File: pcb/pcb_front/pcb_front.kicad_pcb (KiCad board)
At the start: 2 copper layers, 30 x 27 mm, 24 parts, among them J1 MicroLab, J2 LED_BREAKOUT, J3 GAS_BREAKOUT, U1 TBD62783A

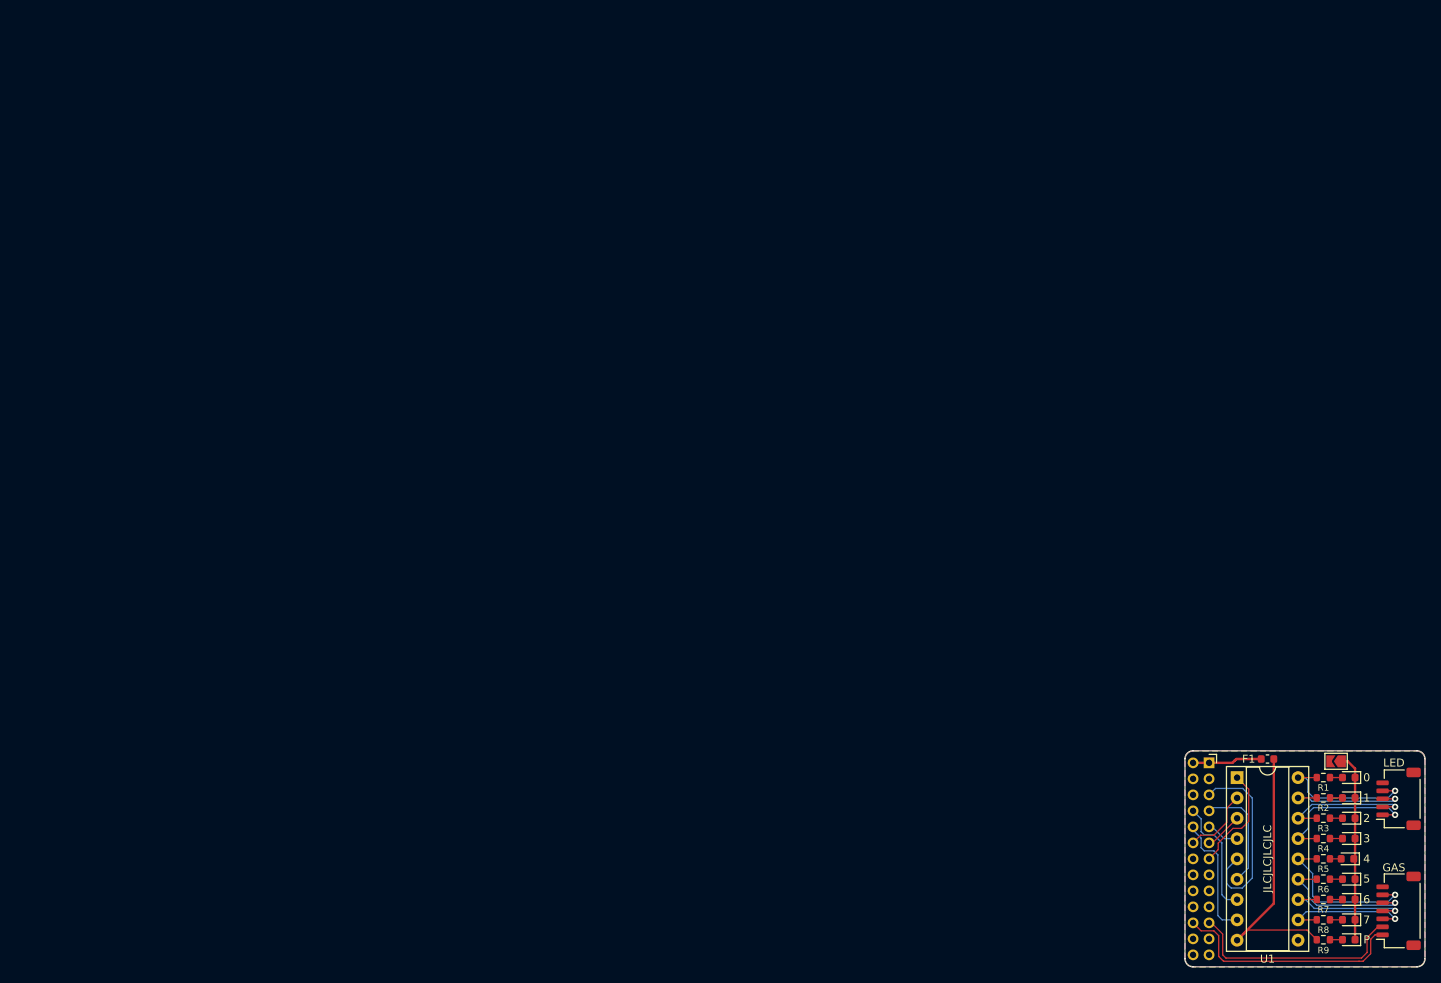
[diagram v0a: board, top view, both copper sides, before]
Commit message: front pcb rev 2
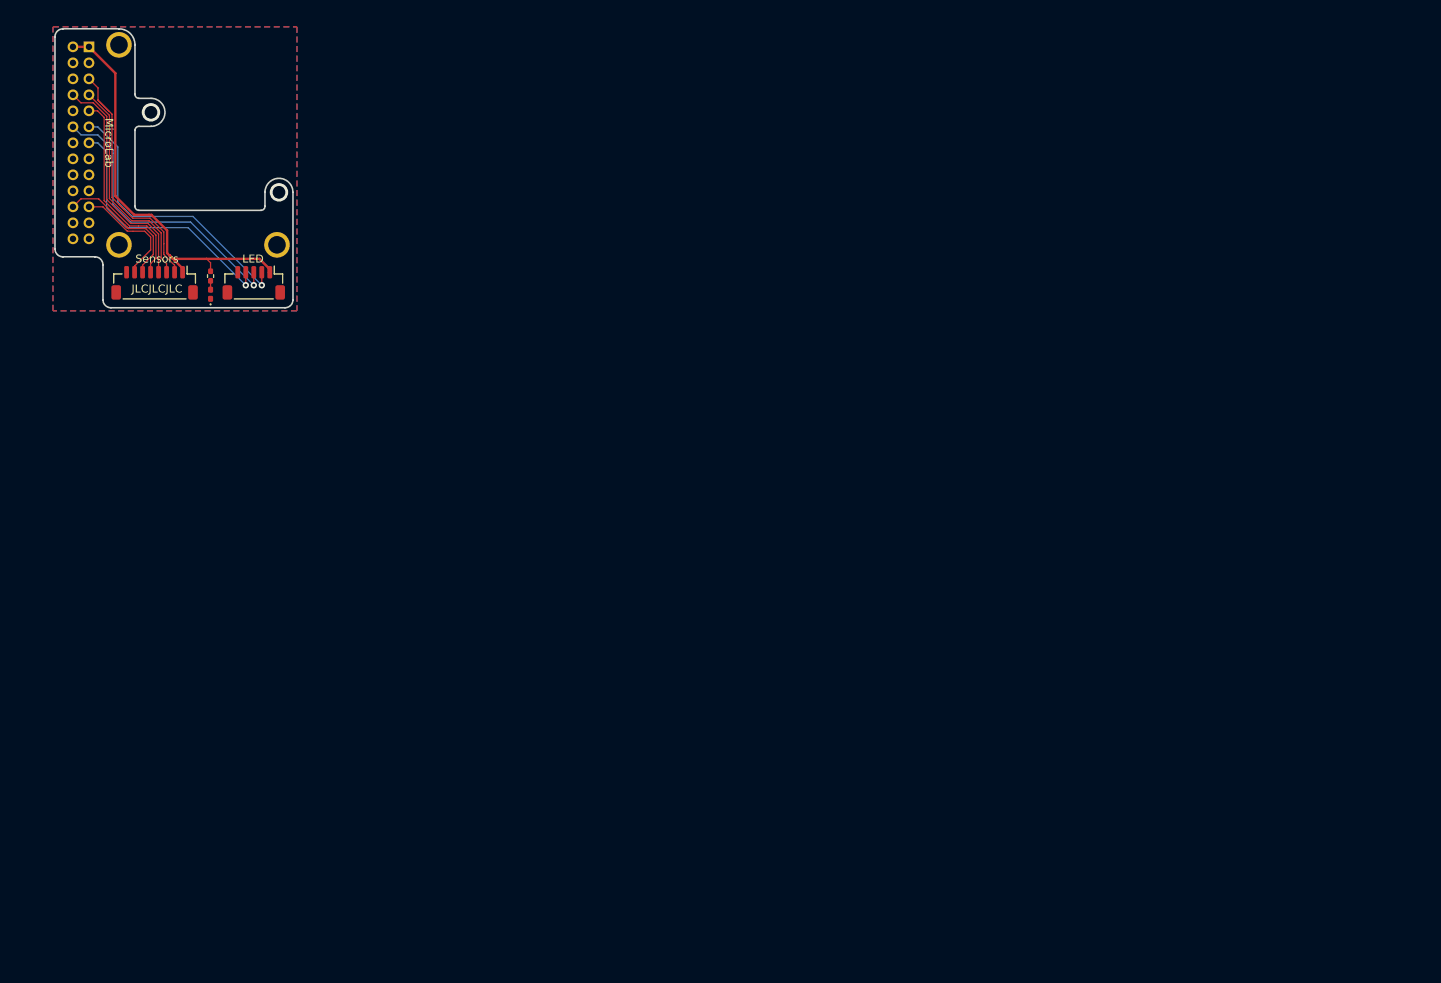
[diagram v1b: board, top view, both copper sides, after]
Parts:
- removed D2: IO1, LED_SMD:LED_0603_1608Metric
- removed D3: IO2, LED_SMD:LED_0603_1608Metric
- removed D4: IO3, LED_SMD:LED_0603_1608Metric
- removed D5: IO4, LED_SMD:LED_0603_1608Metric
- removed D6: IO5, LED_SMD:LED_0603_1608Metric
- removed D7: IO6, LED_SMD:LED_0603_1608Metric
- removed D8: IO7, LED_SMD:LED_0603_1608Metric
- removed D9: PWR, LED_SMD:LED_0603_1608Metric
- removed F1: Polyfuse_Small, Fuse:Fuse_0603_1608Metric
- removed JP1: SolderJumper_2_Open, Jumper:SolderJumper-2_P1.3mm_Open_TrianglePad1.0x1.5mm
- removed R2, R3, R4, R5, R6, R7, R8, R9: 2K, Resistor_SMD:R_0603_1608Metric
- removed U1: TBD62783A, Package_DIP:DIP-18_W7.62mm_Socket
- added H1: M2, MountingHole:MountingHole_2.2mm_M2_DIN965_Pad, F.Cu at (5.75, -0.25)
- added H2: M2, MountingHole:MountingHole_2.2mm_M2_DIN965_Pad, F.Cu at (5.75, 24.8)
- added H3: M2, MountingHole:MountingHole_2.2mm_M2_DIN965_Pad, F.Cu at (25.5, 24.8)
- D1: value IO0 -> LED; footprint LED_SMD:LED_0603_1608Metric -> LED_SMD:LED_0402_1005Metric_Pad0.77x0.64mm_HandSolder
- J1: footprint Connector_PinSocket_2.00mm:PinSocket_2x13_P2.00mm_Horizontal -> Connector_PinHeader_2.00mm:PinHeader_2x13_P2.00mm_Vertical; moved to B.Cu
- J2: value LED_BREAKOUT -> Gas Breakout; footprint Connector_JST:JST_SH_SM05B-SRSS-TB_1x05-1MP_P1.00mm_Horizontal -> Connector_JST:JST_SH_BM08B-SRSS-TB_1x08-1MP_P1.00mm_Vertical
- J3: value GAS_BREAKOUT -> LED Breakout; footprint Connector_JST:JST_SH_SM07B-SRSS-TB_1x07-1MP_P1.00mm_Horizontal -> Connector_JST:JST_SH_BM05B-SRSS-TB_1x05-1MP_P1.00mm_Vertical
- R1: footprint Resistor_SMD:R_0603_1608Metric -> Resistor_SMD:R_0402_1005Metric_Pad0.72x0.64mm_HandSolder
- moved J2 168.3 mm to (10.2, 29.5), turned to 180 degrees
- moved J1 166.2 mm to (2.00, 0.00), turned to 180 degrees
- moved J3 163.2 mm to (22.6, 29.5), turned to 180 degrees
- moved D1 154.6 mm to (17.2, 30.9), turned to 90 degrees
- moved R1 152.6 mm to (17.2, 28.6), turned to 90 degrees
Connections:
- D1 pad 1: Net-(D1-Pad1) -> GND
- J1 pad 1: Net-(J1-Pad1) -> +5V
- J1 pad 2: Net-(J1-Pad1) -> +5V
- J2 pad 1: /V_PUMP_LYO -> +5V
- J2 pad 2: /V_PUMP_CARB -> /IO4
- J2 pad 3: /V_LED_BACT -> /IO5
- J2 pad 4: /V_LED_CAM -> /IO6
- J2 pad 5: GND -> /IO3
- J2 pad MP: (no net) -> GND
- J3 pad 1: /SDA -> +5V
- J3 pad 2: /SCL -> /IO2
- J3 pad 3: /V_FAN -> /IO1
- J3 pad 4: /V_O2 -> /IO0
- J3 pad 5: /V_CO2 -> GND
- J3 pad MP: (no net) -> GND
- R1 pad 2: /V_LED_CAM -> +5V
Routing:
- net /IO2: track 4.79 -> 35.5 mm, vias 0 -> 1
- net /IO1: track 8.87 -> 36.4 mm, vias 0 -> 1
- net Net-(D1-Pad1): track 23.4 -> 0.00 mm
- net /IO3: track 4.11 -> 25.8 mm
- net /V_CH4: track 20.3 -> 0.00 mm, vias 1 -> 0
- net /IO0: track 13.4 -> 32.7 mm, vias 0 -> 1
- net /V_PUMP_LYO: track 19.2 -> 0.00 mm, vias 1 -> 0
- net /V_LED_CAM: track 18.3 -> 0.00 mm, vias 1 -> 0
- net /V_CO2: track 18.0 -> 0.00 mm, vias 1 -> 0
- net +5V: track 34.4 -> 52.2 mm
- net /V_PUMP_CARB: track 16.9 -> 0.00 mm, vias 1 -> 0
- net /V_FAN: track 16.8 -> 0.00 mm, vias 1 -> 0
- net /V_O2: track 16.6 -> 0.00 mm, vias 1 -> 0
- net /V_LED_BACT: track 16.3 -> 0.00 mm, vias 1 -> 0
- net /IO7: track 15.7 -> 0.00 mm
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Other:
- board size 30 x 27 mm -> 29.8 x 34.9 mm
- board text added: "JLCJLCJLC"
- board text added: "LED"
- board text added: "MicroLab"
- board text added: "SAS SpaceLab 2023 Emilio Orcullo"
- board text added: "Sensors"
- board text removed: "JLCJLCJLCJLC"

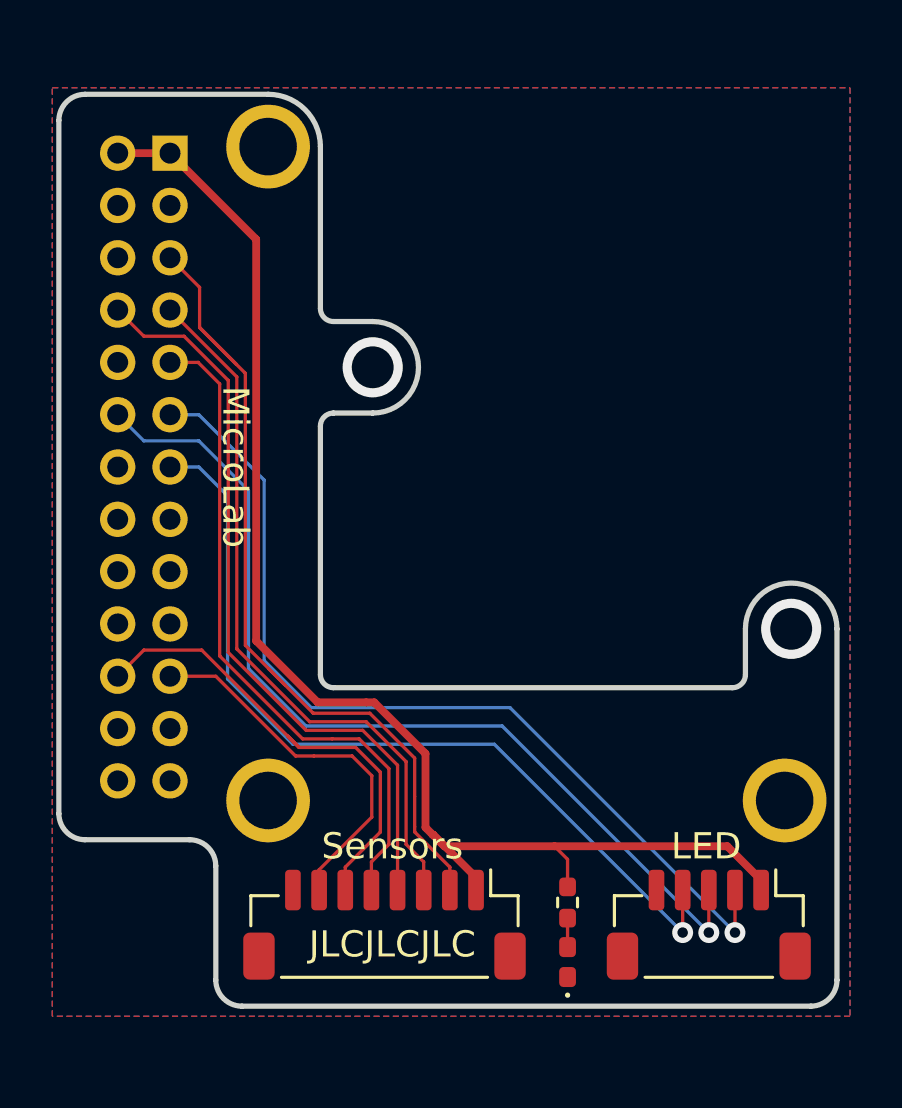
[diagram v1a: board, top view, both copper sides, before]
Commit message: fin
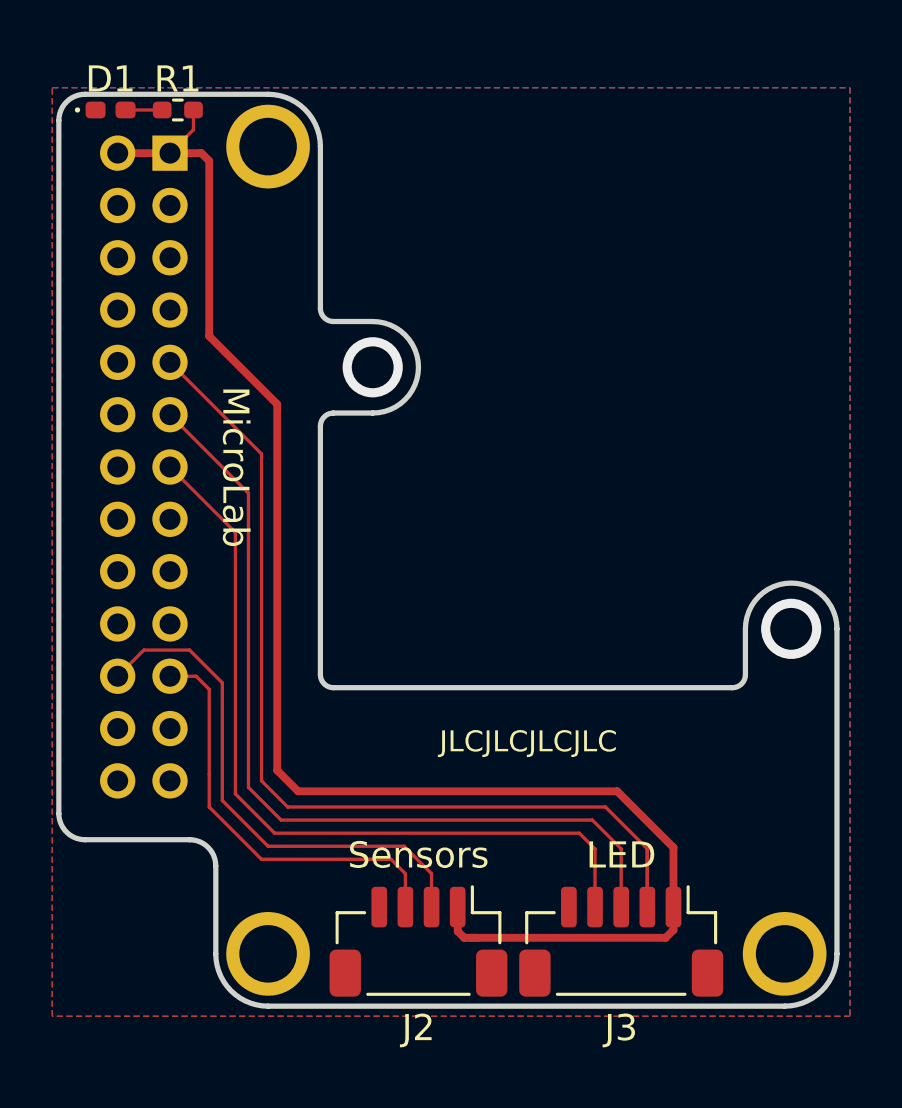
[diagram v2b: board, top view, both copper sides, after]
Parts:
- J2: value Gas Breakout -> Sensors; footprint Connector_JST:JST_SH_BM08B-SRSS-TB_1x08-1MP_P1.00mm_Vertical -> Connector_JST:JST_SH_BM04B-SRSS-TB_1x04-1MP_P1.00mm_Vertical
- J3: value LED Breakout -> LED
- moved D1 37.0 mm to (-0.27, -1.65), turned to 0 degrees
- moved R1 33.8 mm to (2.30, -1.65), turned to 0 degrees
- moved H2 5.86 mm to (5.75, 30.6)
- moved H3 5.86 mm to (25.5, 30.6)
- moved J3 3.41 mm to (19.2, 30.1)
- moved J2 1.45 mm to (11.5, 30.1)
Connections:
- J2 pad 2: /IO4 -> /SDA
- J2 pad 3: /IO5 -> /SCL
- J2 pad 4: /IO6 -> GND
- J3 pad 2: /IO2 -> /IO3
- J3 pad 3: /IO1 -> /IO2
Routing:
- net /IO1: track 36.4 -> 0.00 mm, vias 1 -> 0
- net /IO4: track 32.7 -> 0.00 mm
- net /IO6: track 28.8 -> 0.00 mm
- net /IO5: track 27.5 -> 0.00 mm
- net /IO3: track 25.8 -> 37.8 mm
- net +5V: track 52.2 -> 59.2 mm
- net /IO2: track 35.5 -> 32.9 mm, vias 1 -> 0
- net /IO0: track 32.7 -> 30.4 mm, vias 1 -> 0
- net /SDA: track 18.1 -> 19.9 mm
- net /SCL: track 14.5 -> 16.0 mm
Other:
- outline, holes or cut-outs redrawn
- board text added: "JLCJLCJLCJLC"
- board text added: "SAS SpaceLab 2023"
- board text removed: "JLCJLCJLC"
- board text removed: "SAS SpaceLab 2023 Emilio Orcullo"

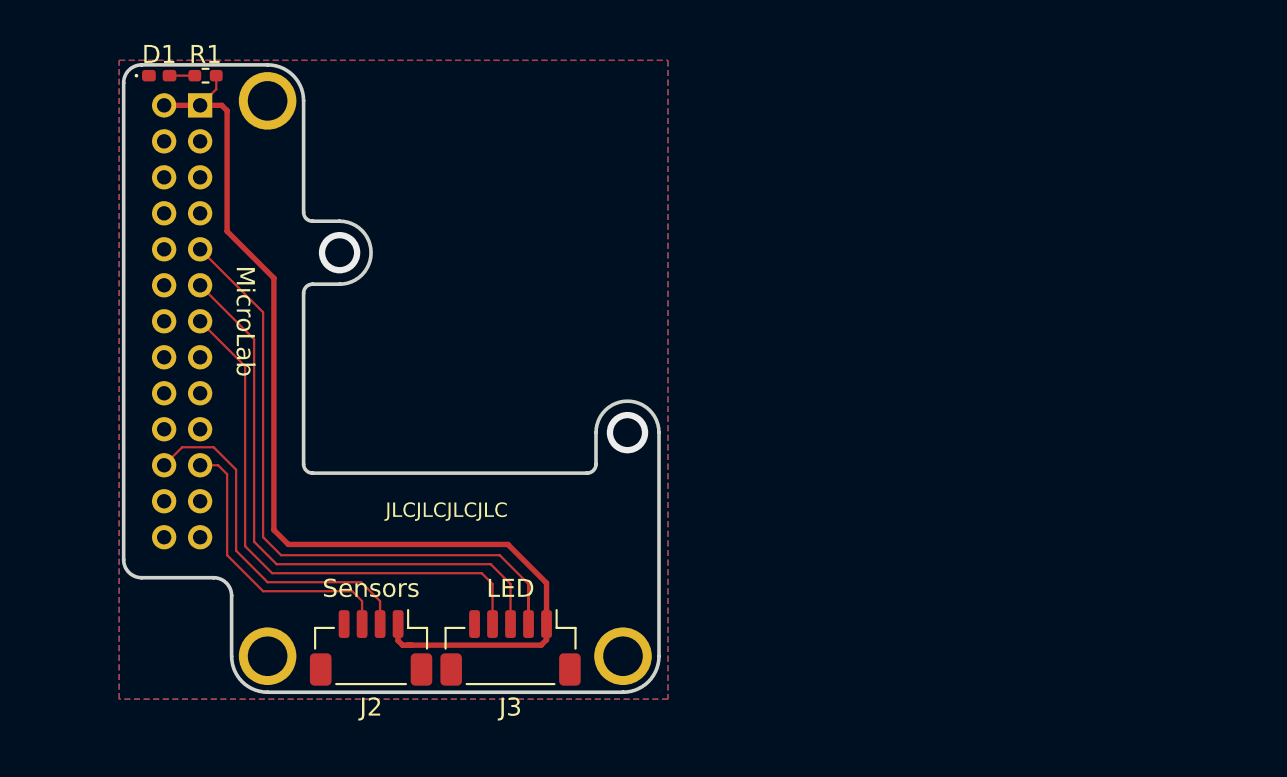
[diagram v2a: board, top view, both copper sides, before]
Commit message: production ver. of PCB
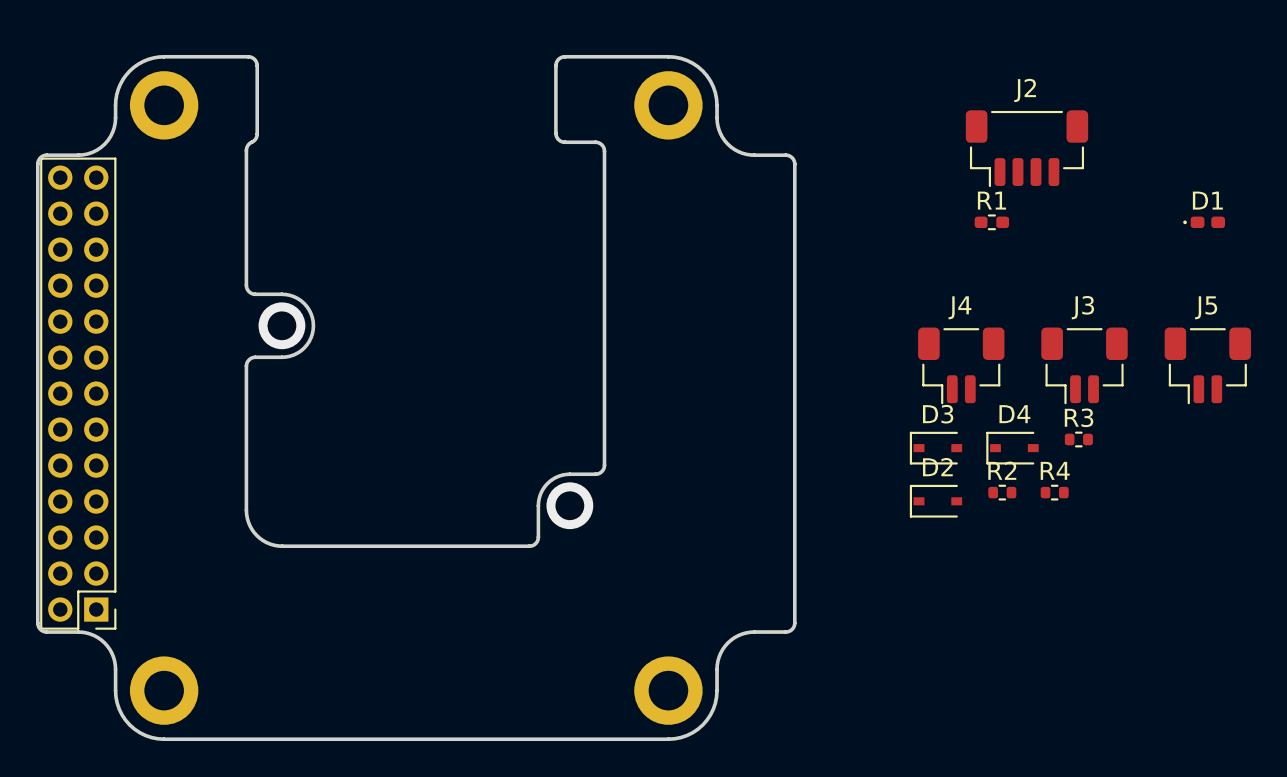
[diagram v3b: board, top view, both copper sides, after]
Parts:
- added D2: D_Small, Diode_SMD:D_SOD-323, F.Cu at (43.0, 22.0)
- added D3: D_Small, Diode_SMD:D_SOD-323, F.Cu at (43.0, 19.1)
- added D4: D_Small, Diode_SMD:D_SOD-323, F.Cu at (47.2, 19.1)
- added H4: M2, MountingHole:MountingHole_2.2mm_M2_DIN965_Pad, F.Cu at (28.0, 32.5)
- added J4: Pump 2, Connector_JST:JST_SH_BM02B-SRSS-TB_1x02-1MP_P1.00mm_Vertical, F.Cu at (44.3, 14.4)
- added J5: LED, Connector_JST:JST_SH_BM02B-SRSS-TB_1x02-1MP_P1.00mm_Vertical, F.Cu at (58.0, 14.4)
- added R2: 10K, Resistor_SMD:R_0402_1005Metric, F.Cu at (46.6, 21.5)
- added R3: 10K, Resistor_SMD:R_0402_1005Metric, F.Cu at (50.8, 18.6)
- added R4: 10K, Resistor_SMD:R_0402_1005Metric, F.Cu at (49.5, 21.5)
- J1: moved to F.Cu
- J3: value LED -> Pump 1; footprint Connector_JST:JST_SH_BM05B-SRSS-TB_1x05-1MP_P1.00mm_Vertical -> Connector_JST:JST_SH_BM02B-SRSS-TB_1x02-1MP_P1.00mm_Vertical
- moved D1 58.8 mm to (58.0, 6.50)
- moved J2 45.8 mm to (48.0, 2.38), turned to 0 degrees
- moved R1 44.5 mm to (46.0, 6.50)
- moved H2 37.9 mm to (28.0, 0.00)
- moved J3 35.6 mm to (51.1, 14.4), turned to 0 degrees
- moved J1 28.6 mm to (-3.77, 28.0)
- moved H3 25.6 mm to (0.00, 32.5)
- moved H1 5.76 mm to (0.00, 0.00)
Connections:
- J3 pad 2: /IO3 -> Net-(D2-Pad2)
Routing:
- net +5V: track 59.2 -> 0.00 mm
- net /IO3: track 37.8 -> 0.00 mm
- net /IO2: track 32.9 -> 0.00 mm
- net /IO0: track 30.4 -> 0.00 mm
- net /SDA: track 19.9 -> 0.00 mm
- net /SCL: track 16.0 -> 0.00 mm
- net Net-(D1-Pad2): track 1.40 -> 0.00 mm
- removed copper zone on B.Cu, net GND
- removed copper zone on F.Cu, net GND
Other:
- board size 29.8 x 34.9 mm -> 42.1 x 37.9 mm
- board text removed: "JLCJLCJLCJLC"
- board text removed: "LED"
- board text removed: "MicroLab"
- board text removed: "SAS SpaceLab 2023"
- board text removed: "Sensors"
